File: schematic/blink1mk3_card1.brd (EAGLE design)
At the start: 14.9 x 9.6 mm, 15 parts, among them U1 EFM32HG309F64G, X2 USBPCB2

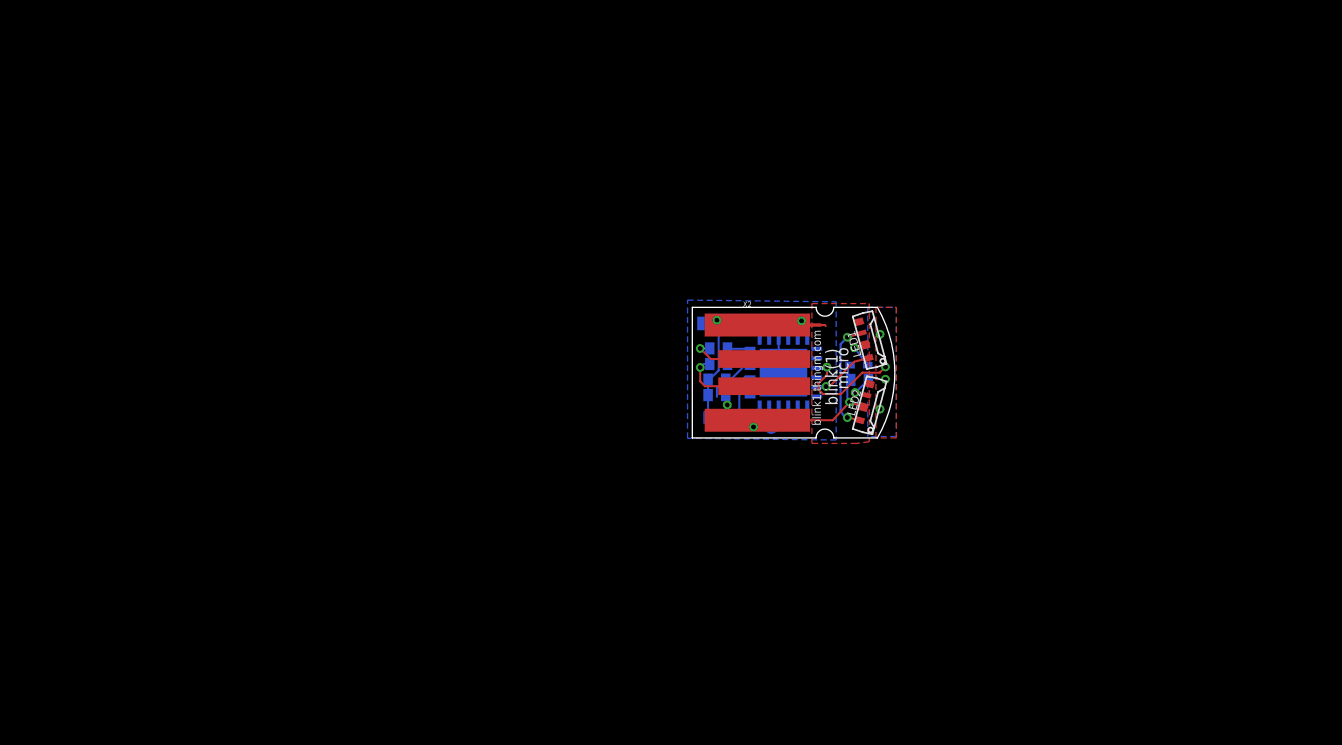
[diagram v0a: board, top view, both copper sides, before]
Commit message: added business card idea
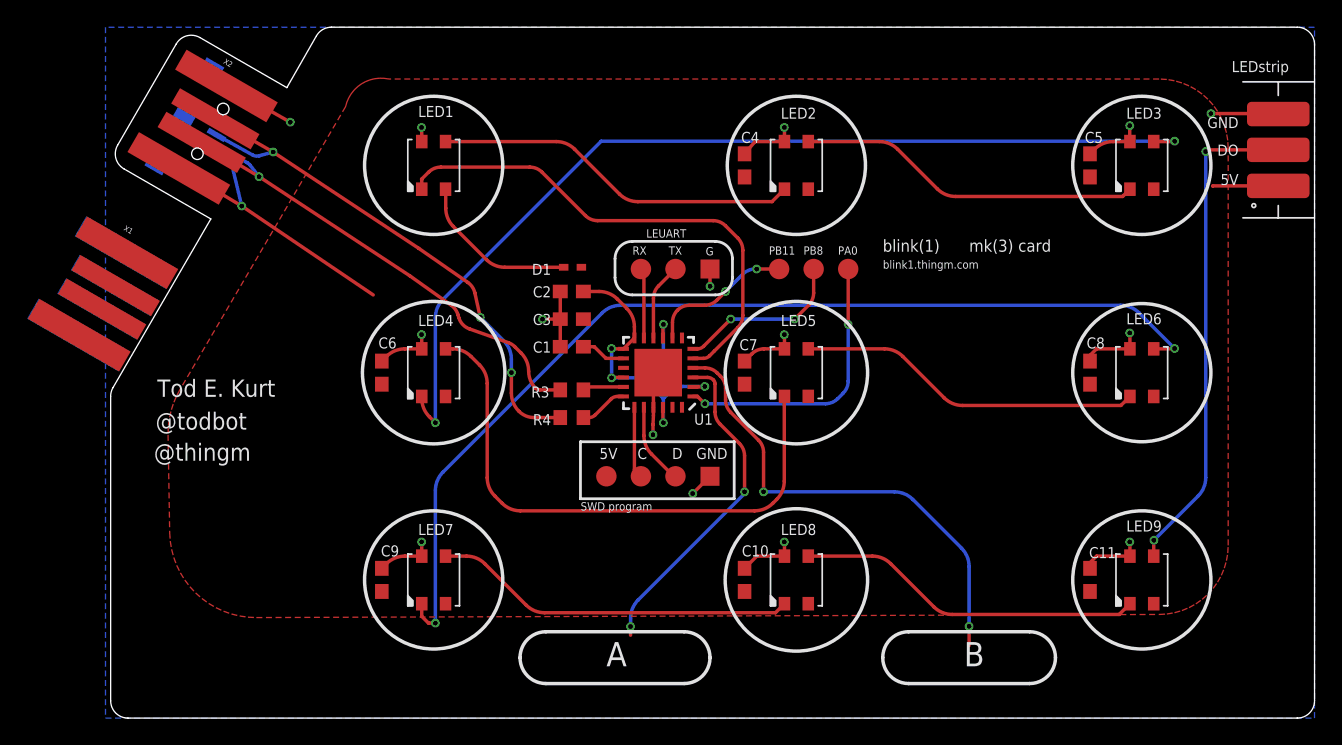
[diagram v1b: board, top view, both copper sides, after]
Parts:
- added C10, C11, C5, C6, C7, C8, C9: 0.1uF, adafruit:C0603
- added GND: TPTP14SQ, testpad:TP14SQ
- added J1: NONPOP, SparkFun-Connectors:USB-B-MICRO-SMD
- added LED3, LED4, LED5, LED6, LED7, LED8, LED9: SK6812MINI, adafruit:LED3535
- added PA0, PB11, PB8, RX, TX: TPTP15R, testpad:TP15R
- added U$1: LED_STRIP_3P, NeoJoints:LEDSTRIP-3P
- added X1, X3: USBPCB2, todstuff:USB-A-PCB-2
- 5V, C, D: value TPTP10R -> TPTP15R; device testpad:TP10R -> testpad:TP15R
- C1, C2, C3, C4: device adafruit:C0402 -> adafruit:C0603
- G: value TPTP10SQ -> TPTP14SQ; device testpad:TP10SQ -> testpad:TP14SQ
- LED1, LED2: value WS2812B4020SIDE -> SK6812MINI; device todstuff:SK6812-SIDE -> adafruit:LED3535
- R3, R4: device adafruit:R0402 -> adafruit:R0603
- moved X2 44.5 mm to (-36.0, 17.3), turned to 330 degrees
- moved LED1 34.6 mm to (-20.3, 15.2), turned to 90 degrees
- moved D1 22.4 mm to (-10.2, 7.75), flipped to the top
- moved LED2 18.5 mm to (6.35, 15.2), turned to 90 degrees
- moved C4 17.9 mm to (2.54, 15.2), flipped to the top, turned to 90 degrees
- moved C 13.4 mm to (-5.08, -7.62), flipped to the top
- moved D 13.3 mm to (-2.54, -7.62), flipped to the top
- moved 5V 12.6 mm to (-7.62, -7.62), flipped to the top
- moved C2 12.5 mm to (-10.2, 5.97), flipped to the top, turned to 180 degrees
- moved C3 12.0 mm to (-10.2, 3.94), flipped to the top, turned to 180 degrees
- moved R4 11.9 mm to (-10.2, -3.30), flipped to the top, turned to 180 degrees
- moved C1 11.9 mm to (-10.2, 1.91), flipped to the top, turned to 180 degrees
- moved R3 11.0 mm to (-10.2, -1.27), flipped to the top, turned to 180 degrees
- moved U1 9.21 mm to (-3.81, 0.00), flipped to the top, turned to 180 degrees
- moved G 4.03 mm to (0.00, 7.62), flipped to the top
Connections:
- removed net LED1: U1.1
- removed net N$1: U1.8
- removed net N$3: U1.6
- new net N$10: LED6.3, LED7.1
- new net N$4: LED7.3, LED8.1
- new net N$5: LED4.3, LED5.1
- new net N$6: LED5.3, LED6.1
- new net N$7: LED2.3, LED3.1
- new net N$8: LED3.3, LED4.1
- new net N$9: LED8.3, LED9.1
- new net PA0: PA0.TP, U1.1
- new net PB11: PB11.TP, U1.8
- new net PB8: PB8.TP, U1.6
- new net VBUS: X1.5V, X3.5V
- net +5V: now also C10.1, C11.1, C5.1, C6.1, C7.1, C8.1, C9.1, J1.VBUS, LED2.2, LED3.2, LED4.2, LED5.2, LED6.2, LED7.2, LED8.2, LED9.2, U$1.A; no longer LED2.1-VDD
- net DI: now also LED1.1; no longer LED1.4-DIN
- net DO: now also LED9.3, U$1.B; no longer LED2.2-DOUT
- net GND: now also C10.2, C11.2, C5.2, C6.2, C7.2, C8.2, C9.2, GND.TP, J1.GND, LED1.4, LED2.4, LED3.4, LED4.4, LED5.4, LED6.4, LED7.4, LED8.4, LED9.4, U$1.C, X1.GND, X3.GND; no longer LED1.3-GND, LED2.3-GND
- net LEUO_RX: now also RX.TP
- net LEUO_TX: now also TX.TP
- net N$2: now also LED1.3, LED2.1; no longer LED1.2-DOUT, LED2.4-DIN
- net USB_D+: now also J1.D+
- net USB_D-: now also J1.D-
- net VLEDA: now also LED1.2; no longer LED1.1-VDD
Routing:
- net N$10: track 0.00 -> 74.9 mm, vias 0 -> 2
- net N$8: track 0.00 -> 71.7 mm, vias 0 -> 2
- net N$5: track 0.00 -> 41.7 mm
- net DO: track 0.00 -> 36.6 mm, vias 0 -> 2
- net CAP1A: track 0.00 -> 35.2 mm, vias 0 -> 2
- net USB_D+: track 5.73 -> 40.5 mm, vias 1 -> 3
- net GND: track 27.2 -> 59.8 mm, vias 3 -> 15
- net DI: track 4.71 -> 37.1 mm, vias 1 -> 0
- net USB_D-: track 6.68 -> 37.3 mm
- net N$4: track 0.00 -> 26.7 mm
- net +3V3: track 3.12 -> 28.9 mm, vias 0 -> 5
- net N$9: track 0.00 -> 25.5 mm
- net N$6: track 0.00 -> 25.4 mm
- net N$7: track 0.00 -> 25.3 mm
- net PA0: track 0.00 -> 20.7 mm, vias 0 -> 2
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- added copper zone on layer 1, net +5V
- added copper zone on layer 1, net CAP1A
- added copper zone on layer 16, net GND
- removed copper zone on layer 16, net +3V3
- removed copper zone on layer 16, net CAP0A
- removed copper zone on layer 1, net GND
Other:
- board size 14.9 x 9.6 mm -> 88.5 x 50.8 mm
- board text added: "5V"
- board text added: "@thingm"
- board text added: "@todbot"
- board text added: "A"
- board text added: "B"
- board text added: "DO"
- board text added: "GND"
- board text added: "Gnd"
- board text added: "LEDstrip"
- board text added: "LEUART"
- board text added: "SWD program"
- board text added: "Tod E. Kurt"
- board text added: "blink1mk3_card"
- board text added: "mk(3) card"
- board text removed: "blink1mk3micro1a"
- board text removed: "micro"
